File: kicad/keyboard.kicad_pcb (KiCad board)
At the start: 2 copper layers, 231 x 116.7 mm, 123 parts, among them SW1 Push, SW10 Push, SW11 Push, SW12 Push, SW14 Push, SW15 Push, SW16 Push, SW17 Push, SW18 Push, SW2 Push, SW20 Push, SW21 Push, SW22 Push, SW23 Push, SW24 Push, SW26 Push, SW27 Push, SW28 Push, SW29 Push, SW3 Push, SW30 Push, SW32 Push, SW33 Push, SW34 Push, SW35 Push, SW38 Push, SW39 Push, SW4 Push, SW40 Push, SW41 Push, SW42 Push, SW44 Push, SW45 Push, SW46 Push, SW47 Push, SW48 Push, SW5 Push, SW50 Push, SW51 Push, SW52 Push, SW53 Push, SW54 Push, SW56 Push, SW57 Push, SW58 Push, SW59 Push, SW6 Push, SW60 Push, SW62 Push, SW63 Push, SW64 Push, SW65 Push, SW66 Push, SW67 Push, SW68 Push, SW69 Push, SW70 Push, SW71 Push, SW72 Push, SW8 Push, SW9 Push, U1 Arduino_Pro_Micro

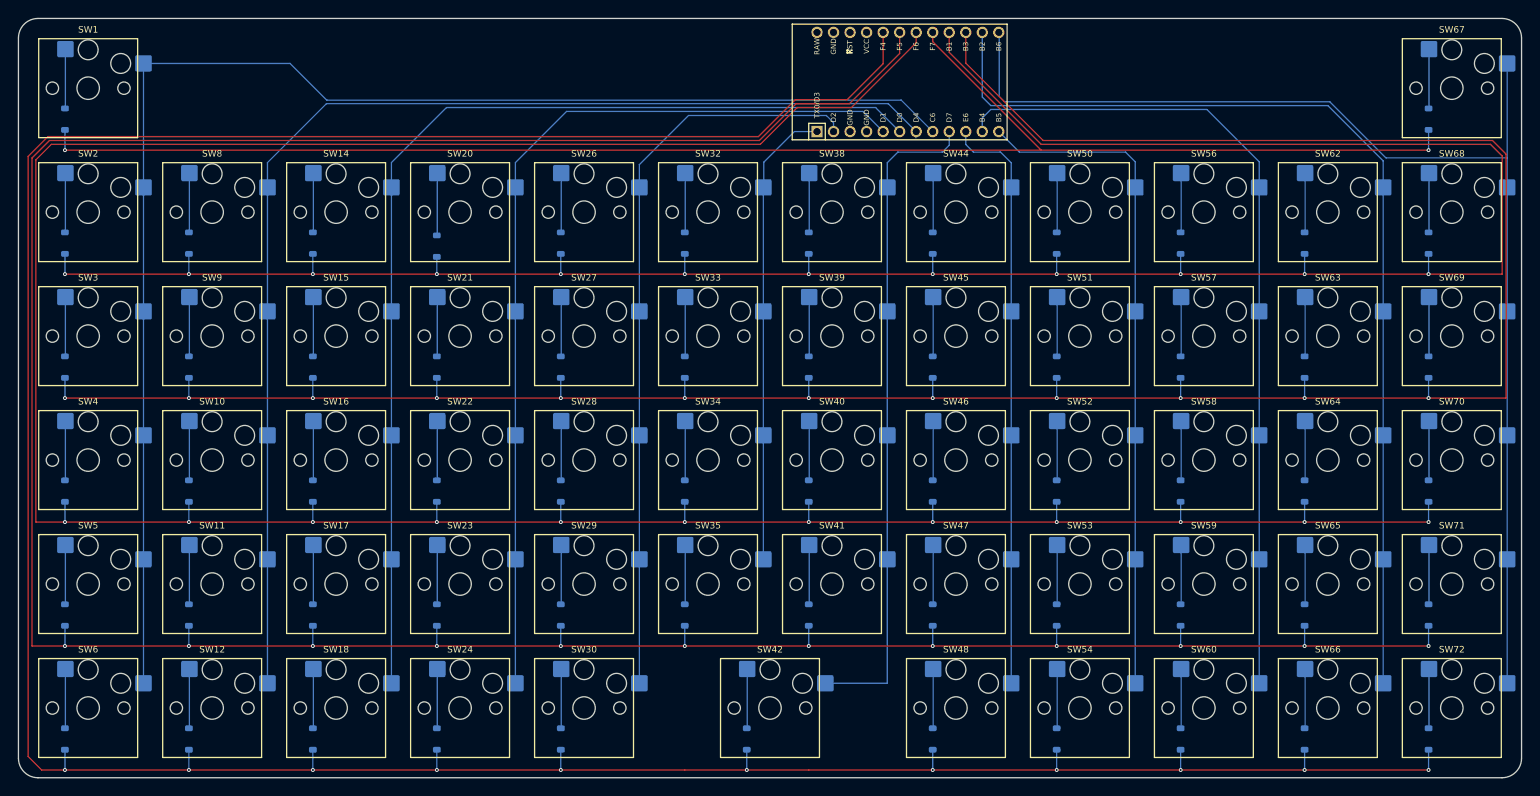
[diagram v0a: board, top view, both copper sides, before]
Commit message: case v1
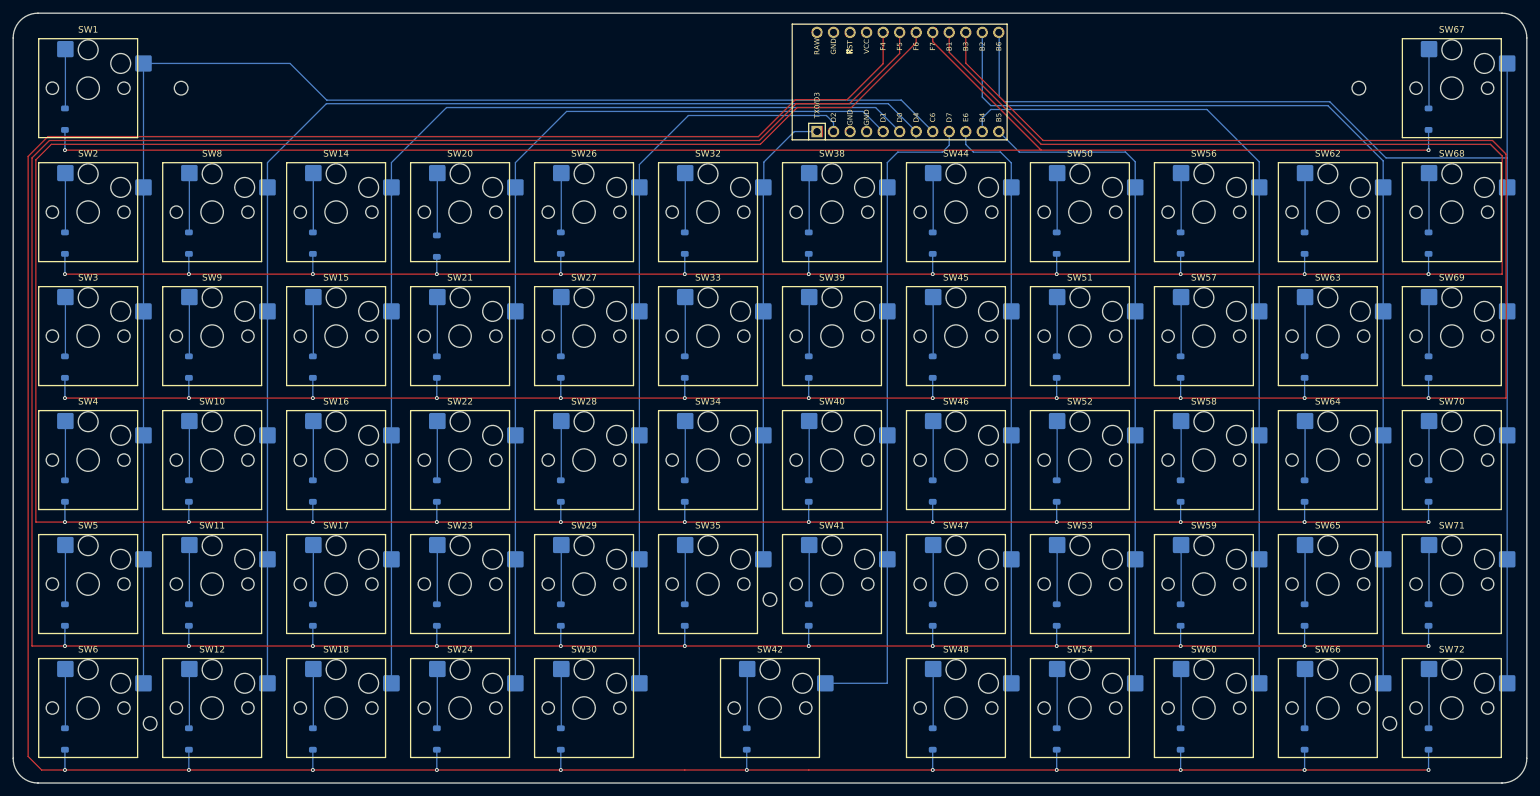
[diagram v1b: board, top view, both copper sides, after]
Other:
- board size 231 x 116.7 mm -> 232.6 x 118.3 mm
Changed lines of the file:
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@@
 	)
 	(gr_line
-		(start 88.571875 183.990625)
-		(end 88.571875 73.309375)
+		(start 87.7625 183.990618)
+		(end 87.7625 73.309368)
+		(stroke
+			(width 0.05)
+			(type default)
+		)
+		(layer "Edge.Cuts")
+	)
+	(gr_circle
+		(center 294.55 81.025)
+		(end 295.6 81.025)
+		(stroke
+			(width 0.05)
+			(type default)
+		)
+		(fill none)
+		(layer "Edge.Cuts")
+	)
+	(gr_circle
+		(center 113.575 81.025)
+		(end 114.625 81.025)
+		(stroke
+			(width 0.05)
+			(type default)
+		)
+		(fill none)
+		(layer "Edge.Cuts")
+	)
+	(gr_circle
+		(center 204.0625 159.60625)
+		(end 205.1125 159.60625)
+		(stroke
+			(width 0.05)
+			(type default)
+		)
+		(fill none)
+		(layer "Edge.Cuts")
+	)
+	(gr_arc
+		(start 320.3625 183.990631)
+		(mid 319.246748 186.684257)
+		(end 316.553118 187.8)
+		(stroke
+			(width 0.05)
+			(type default)
+		)
+		(layer "Edge.Cuts")
+	)
+	(gr_circle
+		(center 299.312324 178.65625)
+		(end 300.362324 178.65625)
+		(stroke
+			(width 0.05)
+			(type default)
+		)
+		(fill none)
+		(layer "Edge.Cuts")
+	)
+	(gr_line
+		(start 91.571875 69.5)
+		(end 316.553125 69.5)
 		(stroke
 			(width 0.05)
@@
 	)
 	(gr_arc
-		(start 319.553125 183.990625)
-		(mid 318.674445 186.111945)
-		(end 316.553125 186.990625)
+		(start 87.7625 73.309368)
+		(mid 88.87825 70.615745)
+		(end 91.571875 69.5)
 		(stroke
 			(width 0.05)
@@
 	)
 	(gr_line
-		(start 91.571875 70.309375)
-		(end 316.553125 70.309375)
+		(start 316.553118 187.8)
+		(end 91.571868 187.8)
 		(stroke
 			(width 0.05)
@@
 	)
 	(gr_arc
-		(start 88.571875 73.309375)
-		(mid 89.450562 71.188062)
-		(end 91.571875 70.309375)
+		(start 316.553132 69.5)
+		(mid 319.246757 70.615752)
+		(end 320.3625 73.309381)
 		(stroke
 			(width 0.05)
@@
 	)
 	(gr_line
-		(start 316.553125 186.990625)
-		(end 91.571875 186.990625)
+		(start 320.3625 73.309381)
+		(end 320.3625 183.990631)
 		(stroke
 			(width 0.05)
@@
 		(layer "Edge.Cuts")
 	)
-	(gr_arc
-		(start 316.553125 70.309375)
-		(mid 318.674445 71.188055)
-		(end 319.553125 73.309375)
+	(gr_circle
+		(center 108.812484 178.65625)
+		(end 109.862484 178.65625)
 		(stroke
 			(width 0.05)
 			(type default)
 		)
-		(layer "Edge.Cuts")
-	)
-	(gr_line
-		(start 319.553125 73.309375)
-		(end 319.553125 183.990625)
-		(stroke
-			(width 0.05)
-			(type default)
-		)
+		(fill none)
 		(layer "Edge.Cuts")
 	)
 	(gr_arc
-		(start 91.571875 186.990625)
-		(mid 89.450555 186.111945)
-		(end 88.571875 183.990625)
+		(start 91.571868 187.8)
+		(mid 88.878242 186.684248)
+		(end 87.7625 183.990618)
 		(stroke
 			(width 0.05)
